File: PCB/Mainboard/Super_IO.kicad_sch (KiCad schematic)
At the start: 1 part, among them U22 FDC37C665IR

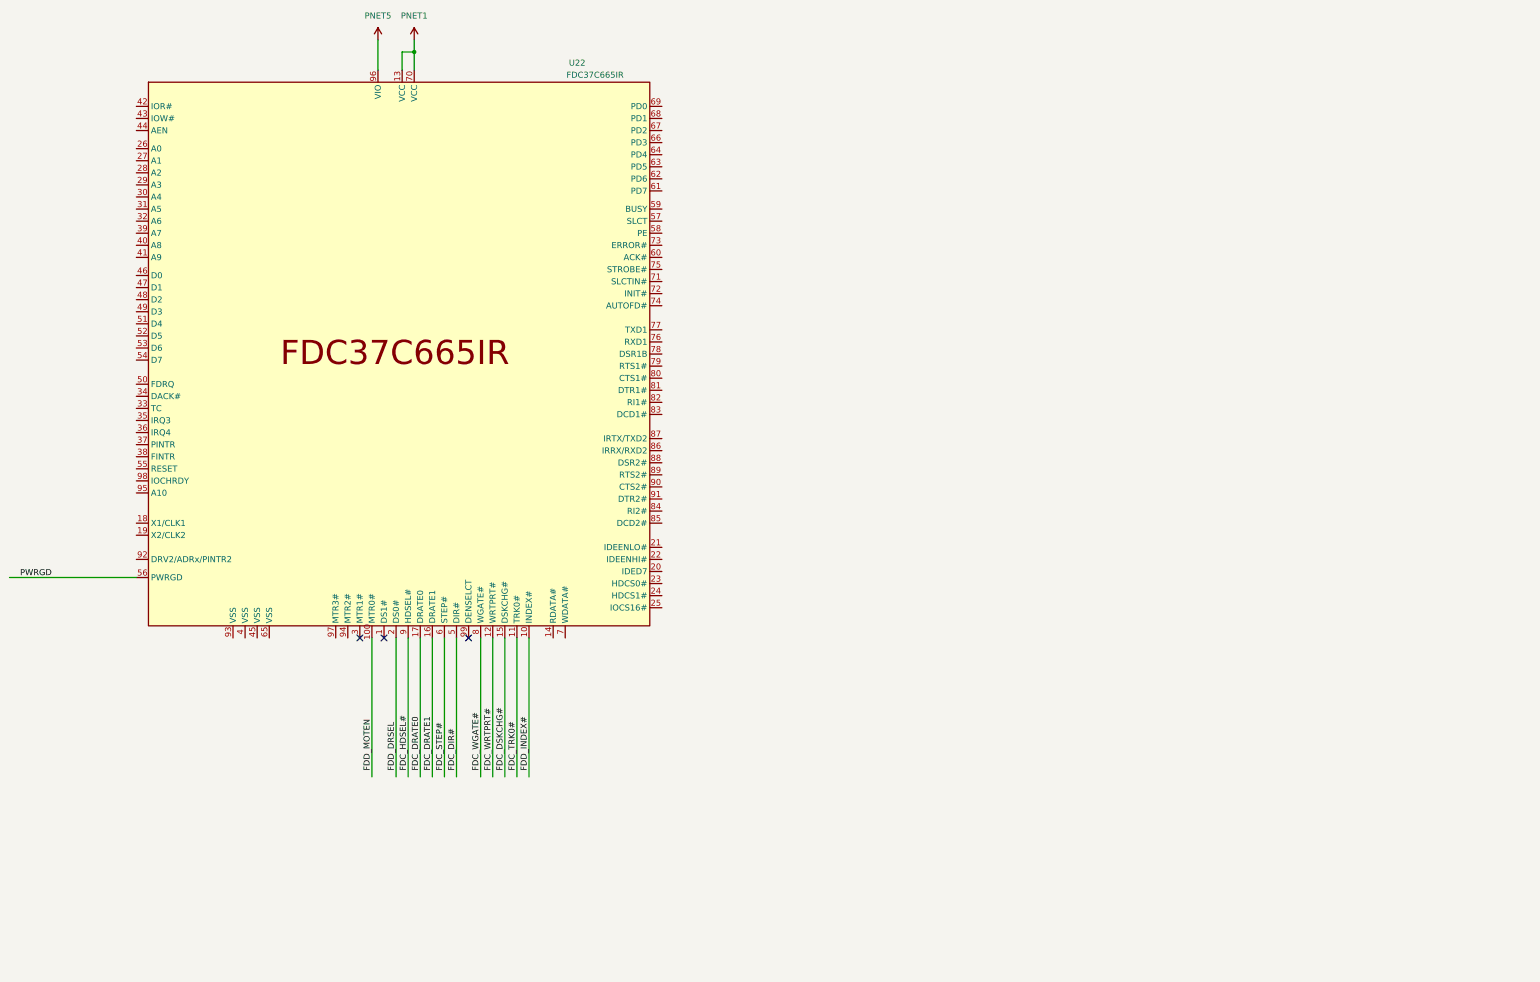
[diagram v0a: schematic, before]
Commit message: Add files via upload
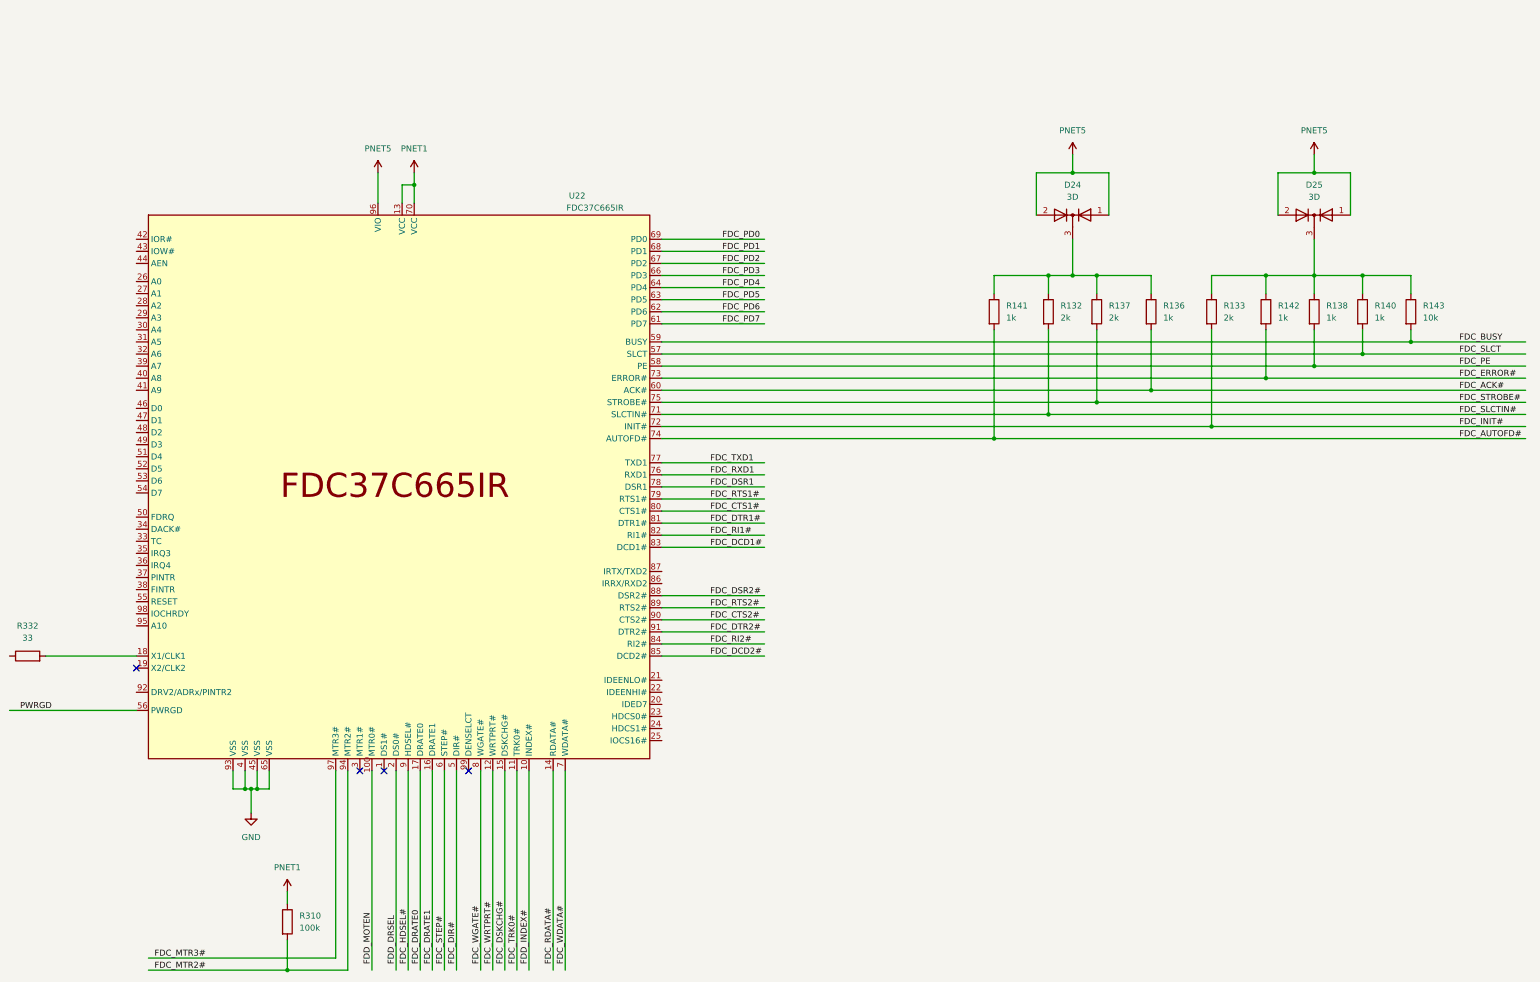
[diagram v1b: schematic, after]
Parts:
- added D24, D25: 3D, symbol Device:D_Dual_CommonCathode_AKA
- added R132, R133, R137: 2k, symbol Device:R
- added R136, R138, R140, R141, R142: 1k, symbol Device:R
- added R143: 10k, symbol Device:R
- added R310: 100k, symbol Device:R
- added R332: 33, symbol Device:R
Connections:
- net PNET1: now also R310.1
- net PNET5: now also D24.1 (A), D24.2 (A), D25.1 (A), D25.2 (A)
- net FDC_RDATA#: now reaches U22.14 (RDATA#)
- net at U22.18 (X1/CLK1): now also R332.2
- net GND: now reaches U22.4 (VSS)
- net GND: now also U22.45 (VSS), U22.65 (VSS), U22.93 (VSS)
- net FDC_SLCT: now reaches U22.57 (SLCT)
- net FDC_SLCT: now also R140.2
- net FDC_PE: now reaches U22.58 (PE)
- net FDC_PE: now also R138.2
- net FDC_BUSY: now reaches U22.59 (BUSY)
- net FDC_BUSY: now also R143.2
- net FDC_ACK#: now reaches U22.60 (ACK#)
- net FDC_ACK#: now also R136.2
- net FDC_PD7: now reaches U22.61 (PD7)
- net FDC_PD6: now reaches U22.62 (PD6)
- net FDC_PD5: now reaches U22.63 (PD5)
- net FDC_PD4: now reaches U22.64 (PD4)
- net FDC_PD3: now reaches U22.66 (PD3)
- net FDC_PD2: now reaches U22.67 (PD2)
- net FDC_PD1: now reaches U22.68 (PD1)
- net FDC_PD0: now reaches U22.69 (PD0)
- net FDC_WDATA#: now reaches U22.7 (WDATA#)
- net FDC_SLCTIN#: now reaches U22.71 (SLCTIN#)
- net FDC_SLCTIN#: now also R132.2
- net FDC_INIT#: now reaches U22.72 (INIT#)
- net FDC_INIT#: now also R133.2
- net FDC_ERROR#: now reaches U22.73 (ERROR#)
- net FDC_ERROR#: now also R142.2
- net FDC_AUTOFD#: now reaches U22.74 (AUTOFD#)
- net FDC_AUTOFD#: now also R141.2
- net FDC_STROBE#: now reaches U22.75 (STROBE#)
- net FDC_STROBE#: now also R137.2
- net FDC_RXD1: now reaches U22.76 (RXD1)
- net FDC_TXD1: now reaches U22.77 (TXD1)
- net FDC_DSR1: now reaches U22.78 (DSR1)
- net FDC_RTS1#: now reaches U22.79 (RTS1#)
- net FDC_CTS1#: now reaches U22.80 (CTS1#)
- net FDC_DTR1#: now reaches U22.81 (DTR1#)
- net FDC_RI1#: now reaches U22.82 (RI1#)
- net FDC_DCD1#: now reaches U22.83 (DCD1#)
- net FDC_RI2#: now reaches U22.84 (RI2#)
- net FDC_DCD2#: now reaches U22.85 (DCD2#)
- net FDC_DSR2#: now reaches U22.88 (DSR2#)
- net FDC_RTS2#: now reaches U22.89 (RTS2#)
- net FDC_CTS2#: now reaches U22.90 (CTS2#)
- net FDC_DTR2#: now reaches U22.91 (DTR2#)
- net FDC_MTR2#: now reaches U22.94 (MTR2#)
- net FDC_MTR2#: now also R310.2
- net FDC_MTR3#: now reaches U22.97 (MTR3#)
- new net: D25.3 (K), R133.1, R138.1, R140.1, R142.1, R143.1
- new net: D24.3 (K), R132.1, R136.1, R137.1, R141.1
- no-connect marks 3 -> 4
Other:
- moved on the sheet: U22
